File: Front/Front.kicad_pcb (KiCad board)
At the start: 2 copper layers, 40 x 40 mm, 42 parts, among them J1 USB_B_Micro, Q1 BC849, Q2 BC849, SW2 SW_Push, U1 CH340C, U10 ESP32-WROOM-32, U2 CJVL53L0XV2, U3 SPX3819M5-L-3-3

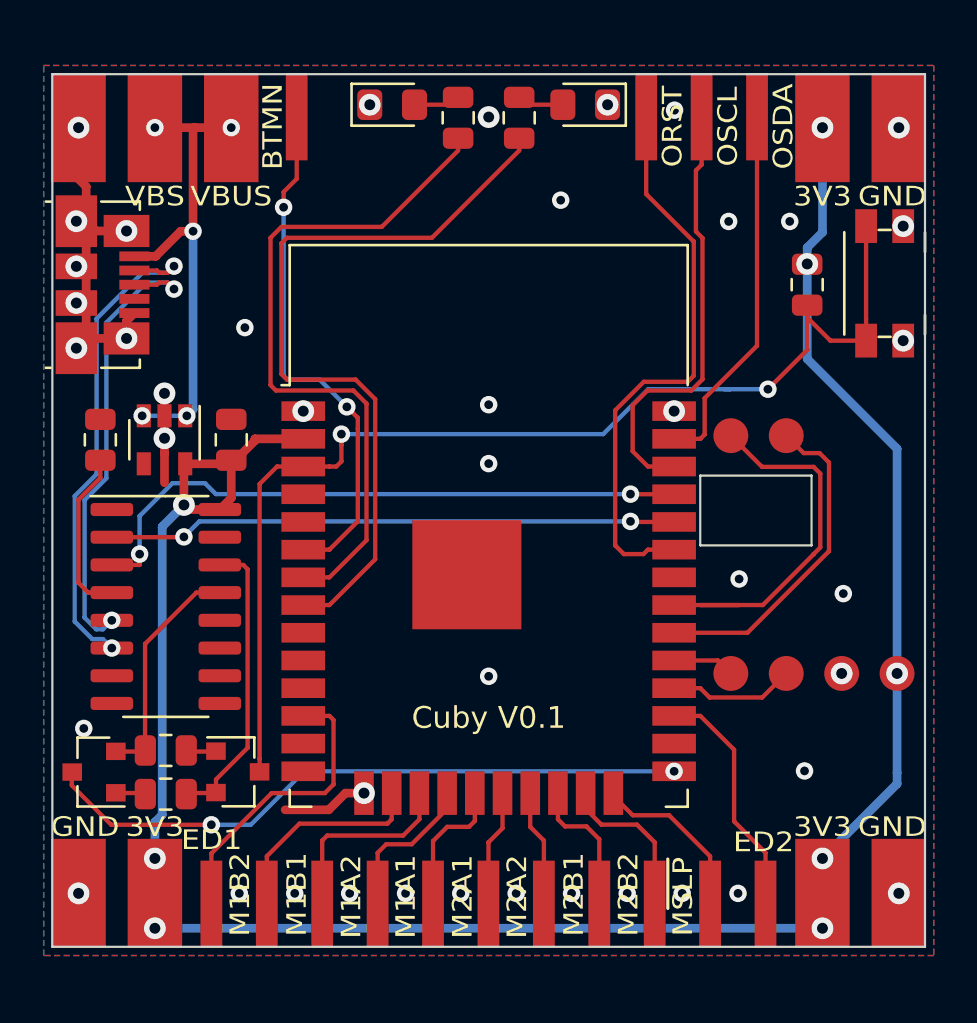
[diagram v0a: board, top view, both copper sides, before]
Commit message: V0.2: Redo front schematic and PCB
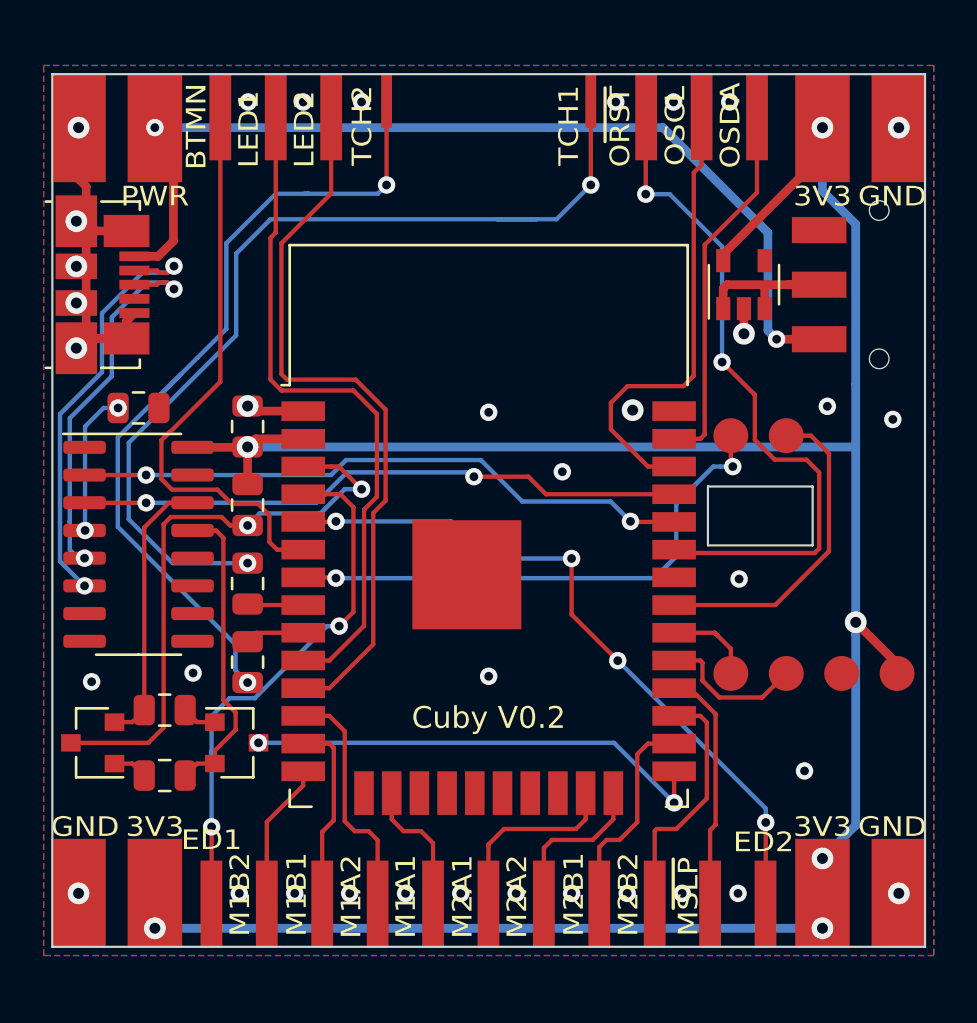
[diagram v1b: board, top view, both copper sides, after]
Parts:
- removed D1: BLUE, LED_SMD:LED_0805_2012Metric_Pad1.15x1.40mm_HandSolder
- removed D2: GREEN, LED_SMD:LED_0805_2012Metric_Pad1.15x1.40mm_HandSolder
- removed G***: LOGO, Print:d1
- removed H17: VBS, Custom:Mounting_Pad_Power
- removed SW2: SW_Push, Button_Switch_SMD:Panasonic_EVQPUJ_EVQPUA
- added H25: LED1, Custom:Mounting_Pad_Signal, F.Cu at (205.7, 105.0)
- added H26: LED2, Custom:Mounting_Pad_Signal, F.Cu at (208.3, 105.0)
- added H27: TCH2, Custom:Mounting_Pad_Touch, F.Cu at (210.8, 104.2)
- added H28: TCH1, Custom:Mounting_Pad_Touch, F.Cu at (220.2, 104.2)
- added SW1: SW_DPDT_x2, Custom:JS102011SAQN, F.Cu at (230.7, 112.7)
- H1: value VBUS -> PWR
- H16: value ORST -> O~RST
- R3, R4: value 150 -> 510
- moved R18 27.6 mm to (204.4, 122.8)
- moved U3 27.5 mm to (227.2, 112.7), turned to 90 degrees
- moved R4 26.8 mm to (204.4, 129.9), turned to 90 degrees
- moved R3 24.7 mm to (204.4, 126.3), turned to 90 degrees
- moved Q1 6.78 mm to (197.3, 133.7), turned to 180 degrees
- moved Q2 6.68 mm to (203.9, 133.7), turned to 0 degrees
- moved R2 3.85 mm to (200.7, 132.2), turned to 180 degrees
- moved H1 3.50 mm to (200.2, 105.5)
- moved H11 3.50 mm to (203.2, 105.0)
- moved U1 3.11 mm to (199.4, 124.5)
- moved C1 2.28 mm to (199.4, 118.3), turned to 0 degrees
- moved R1 1.15 mm to (200.7, 135.2), turned to 180 degrees
- moved C2 0.97 mm to (204.4, 119.2)
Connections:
- R3 pad 1: Net-(D1-Pad2) -> /TOUCH1
- R3 pad 2: /STATUS_LED_BLUE -> Net-(H28-Pad1)
- R4 pad 2: /STATUS_LED_GRN -> /TOUCH2
- U10 pad 10: (no net) -> /LED1
- U10 pad 11: (no net) -> /LED2
- U10 pad 12: /ED_IN1 -> /M1_AOUT2
- U10 pad 13: (no net) -> /M1_BOUT1
- U10 pad 14: (no net) -> /M1_BOUT2
- U10 pad 16: /M1_BOUT2 -> /M1_AOUT1
- U10 pad 17: /M1_BOUT1 -> (no net)
- U10 pad 18: /M1_AOUT2 -> (no net)
- U10 pad 19: /M1_AOUT1 -> (no net)
- U10 pad 20: /M2_AOUT1 -> (no net)
- U10 pad 21: /M2_AOUT2 -> (no net)
- U10 pad 22: /M2_BOUT1 -> (no net)
- U10 pad 23: /M2_BOUT2 -> /M2_AOUT1
- U10 pad 24: /M1_M2_~SLEEP -> /M2_AOUT2
- U10 pad 26: (no net) -> /M2_BOUT1
- U10 pad 27: /ED_IN2 -> /M2_BOUT2
- U10 pad 28: /OD_SCL -> /M1_M2_~SLEEP
- U10 pad 29: /OD_SDA -> /OD_SCL
- U10 pad 30: /OD_SHUT -> /OD_SDA
- U10 pad 31: /OD_INTERRUPT -> /OD_SHUT
- U10 pad 4: (no net) -> /ED_IN1
- U10 pad 5: (no net) -> /ED_IN2
- U10 pad 7: /STATUS_LED_GRN -> /OD_INTERRUPT
- U10 pad 8: /STATUS_LED_BLUE -> /TOUCH1
- U10 pad 9: (no net) -> /TOUCH2
- U3 pad 1: VBUS -> Net-(SW1-Pad2)
- U3 pad 3: VBUS -> Net-(SW1-Pad2)
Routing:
- net Net-(H28-Pad1): track 0.00 -> 43.8 mm, vias 0 -> 2
- net Net-(H27-Pad1): track 2.14 -> 38.5 mm, vias 0 -> 2
- net /STATUS_LED_BLUE: track 35.8 -> 0.00 mm
- net /LED2: track 0.00 -> 33.2 mm
- net /STATUS_LED_GRN: track 32.2 -> 0.00 mm
- net /LED1: track 0.00 -> 31.1 mm
- net /~RST: track 52.8 -> 27.0 mm
- net VBUS: track 21.9 -> 44.7 mm, vias 5 -> 2
- net /ED_IN2: track 11.1 -> 32.6 mm, vias 0 -> 4
- net +3V3: track 96.7 -> 111.3 mm, vias 8 -> 6
- net /ED_IN1: track 15.2 -> 26.5 mm, vias 0 -> 2
- net /GPIO0: track 30.0 -> 21.6 mm
- net /OD_INTERRUPT: track 17.7 -> 25.8 mm, vias 0 -> 2
- net Net-(SW1-Pad2): track 0.00 -> 7.93 mm
- net GND: track 27.1 -> 20.2 mm, vias 43 -> 36
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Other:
- outline, holes or cut-outs redrawn
- board text added: "Cuby V0.2"
- board text removed: "Cuby V0.1"
